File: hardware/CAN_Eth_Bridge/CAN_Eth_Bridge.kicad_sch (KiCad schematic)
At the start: 25 parts, among them J102 Global LV and CAN, J105 Conn_02x05_Odd_Even, J106 uart, SW101 SW_Push, U101 MCP2542FDxMF, U103 XMSM0G3507SDGS28R

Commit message: long 88 can stick
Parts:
- removed F101: ~1A, Fuse:Fuseholder_Blade_Mini_Keystone_3568, symbol Device:Fuse_Small
- removed J105: Conn_02x05_Odd_Even, Connector_PinHeader_1.27mm:PinHeader_2x05_P1.27mm_Vertical_SMD, symbol Connector_Generic:Conn_02x05_Odd_Even
- removed J106: uart, Connector_PinHeader_2.54mm:PinHeader_1x03_P2.54mm_Vertical, symbol Connector:Conn_01x03_Pin
- added C101, C102, C103: 220n, Capacitor_SMD:C_0805_2012Metric_Pad1.18x1.45mm_HandSolder, symbol Device:C_Small
- added D101: TS4148, Diode_SMD:D_0805_2012Metric_Pad1.15x1.40mm_HandSolder, symbol Device:D_Small
- added FL102: Choke_CommonMode_FerriteCore_1243, Inductor_SMD:L_CommonModeChoke_Coilcraft_1812CAN, symbol Filter:Choke_CommonMode_FerriteCore_1243
- added J101: Conn_01x05_Pin, Connector_PinHeader_2.54mm:PinHeader_1x05_P2.54mm_Vertical, symbol Connector:Conn_01x05_Pin
- added SW102: SW_DIP_x06, Button_Switch_SMD:SW_DIP_SPSTx06_Slide_Copal_CHS-06B_W7.62mm_P1.27mm, symbol Switch:SW_DIP_x06
- added U102: AP7384-50SA, Package_TO_SOT_SMD:SOT-23-3, symbol Regulator_Linear:AP7384-50SA
- added U104: AP7381-33SA-7, Package_TO_SOT_SMD:SOT-23, symbol Regulator_Linear:AP7381-33SA-7
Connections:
- net GLV- is gone; now on net GND: J102.2 (Pin_2)
- net +3.3V: now also U103.7 (VDD), C101.1, U104.2 (VO)
- net +5V: now also C102.1, U102.2 (VO)
- net GLV+: now also D101.2 (A)
- net GND: now also U103.8 (VSS), C101.2, C102.2, C103.2, J101.1 (Pin_1), U102.3 (GND), U104.3 (GND)
- net G_CAN+: now also FL102.1; no longer U101.7 (CANH)
- net G_CAN-: now also FL102.4; no longer U101.6 (CANL)
- net XDS_RXD: now also J101.3 (Pin_3)
- net XDS_TCK_SWDCLK: now also U103.23 (PA20/SWCLK), J101.5 (Pin_5)
- net XDS_TMS_SWDIO: now also U103.22 (PA19/SWDIO), J101.4 (Pin_4)
- net XDS_TXD: now also J101.2 (Pin_2)
- net vcore: now also U103.3 (VCORE)
- net at R112.1, SW101.1: now also U103.6 (NRST)
- net at U103.9 (PA2_/_ROSC): now also R111.2
- new net: C103.1, D101.1 (K), U102.1 (VI), U104.1 (VI)
- new net: FL102.3, U101.6 (CANL)
- new net: FL102.2, U101.7 (CANH)
- no-connect marks 4 -> 0
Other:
- removed sheet GLV PSU
- note added: "PSU"
- note removed: "- LV only. no HV present - (10,35]VDC GLV working - swap relays for >12VDC operation - IL assumed to share GLV GND - IL sense diode set for ~12VDC"
- note removed: "PWR"
- note removed: "SWD fish"
- moved on the sheet: C104, D103, D104, D105, D106, J102, R107, R108, R109, R110, U101, U103

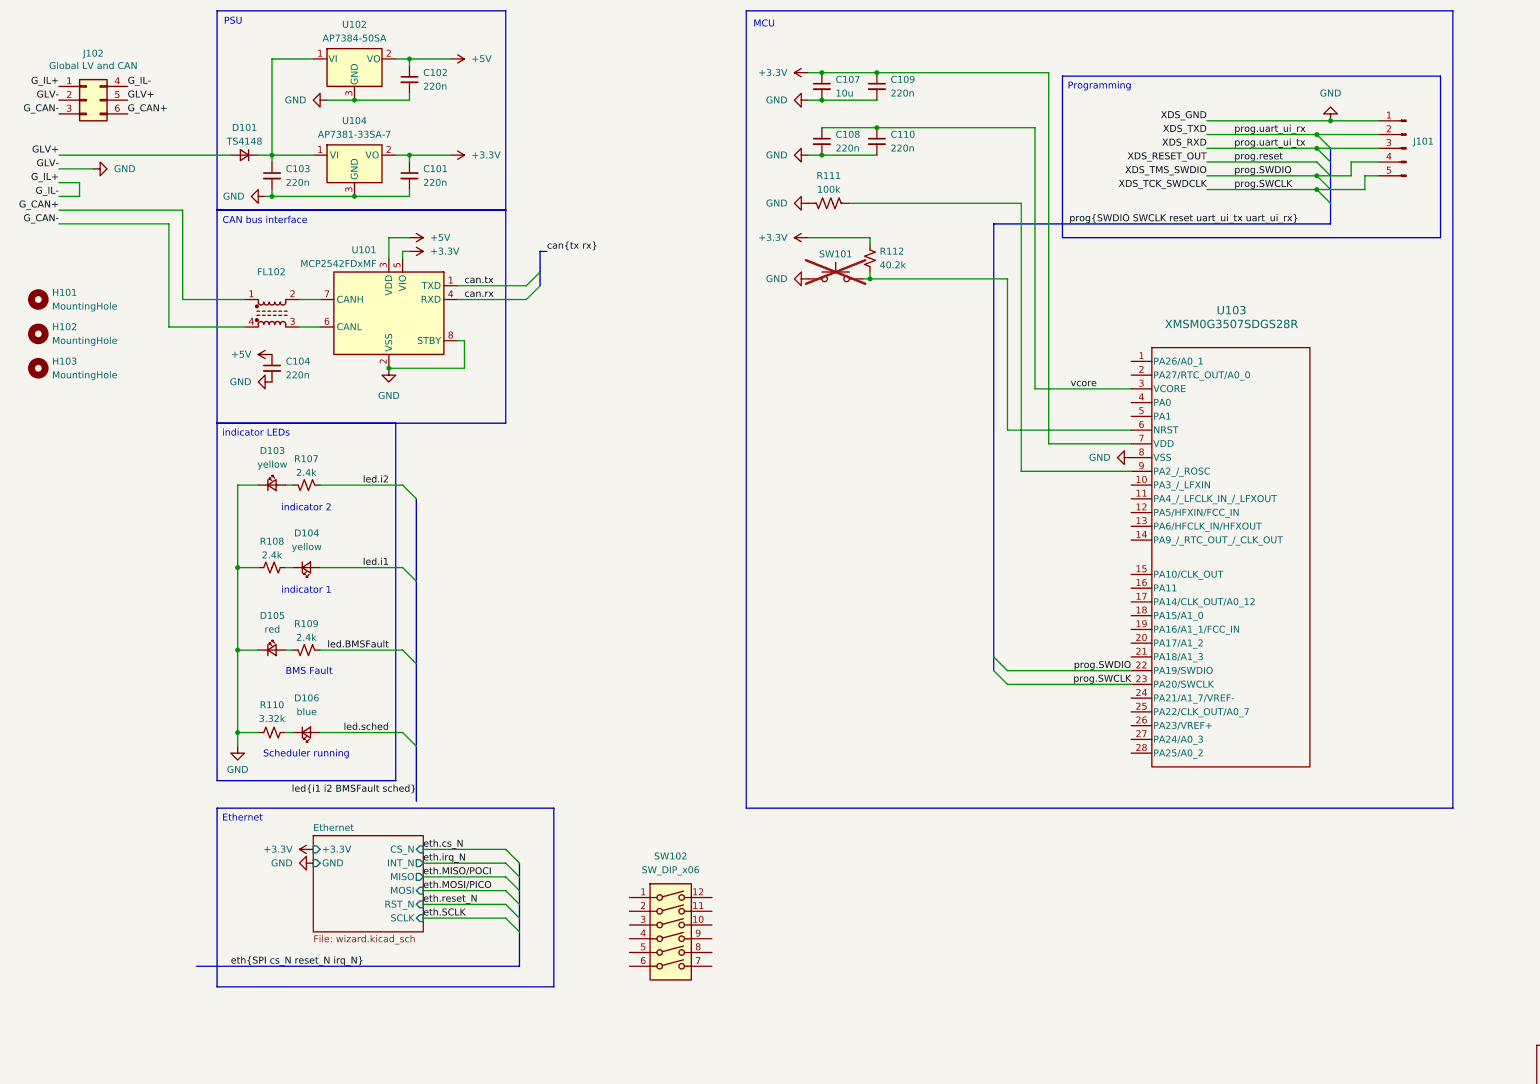
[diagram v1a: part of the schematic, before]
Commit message: shuffled
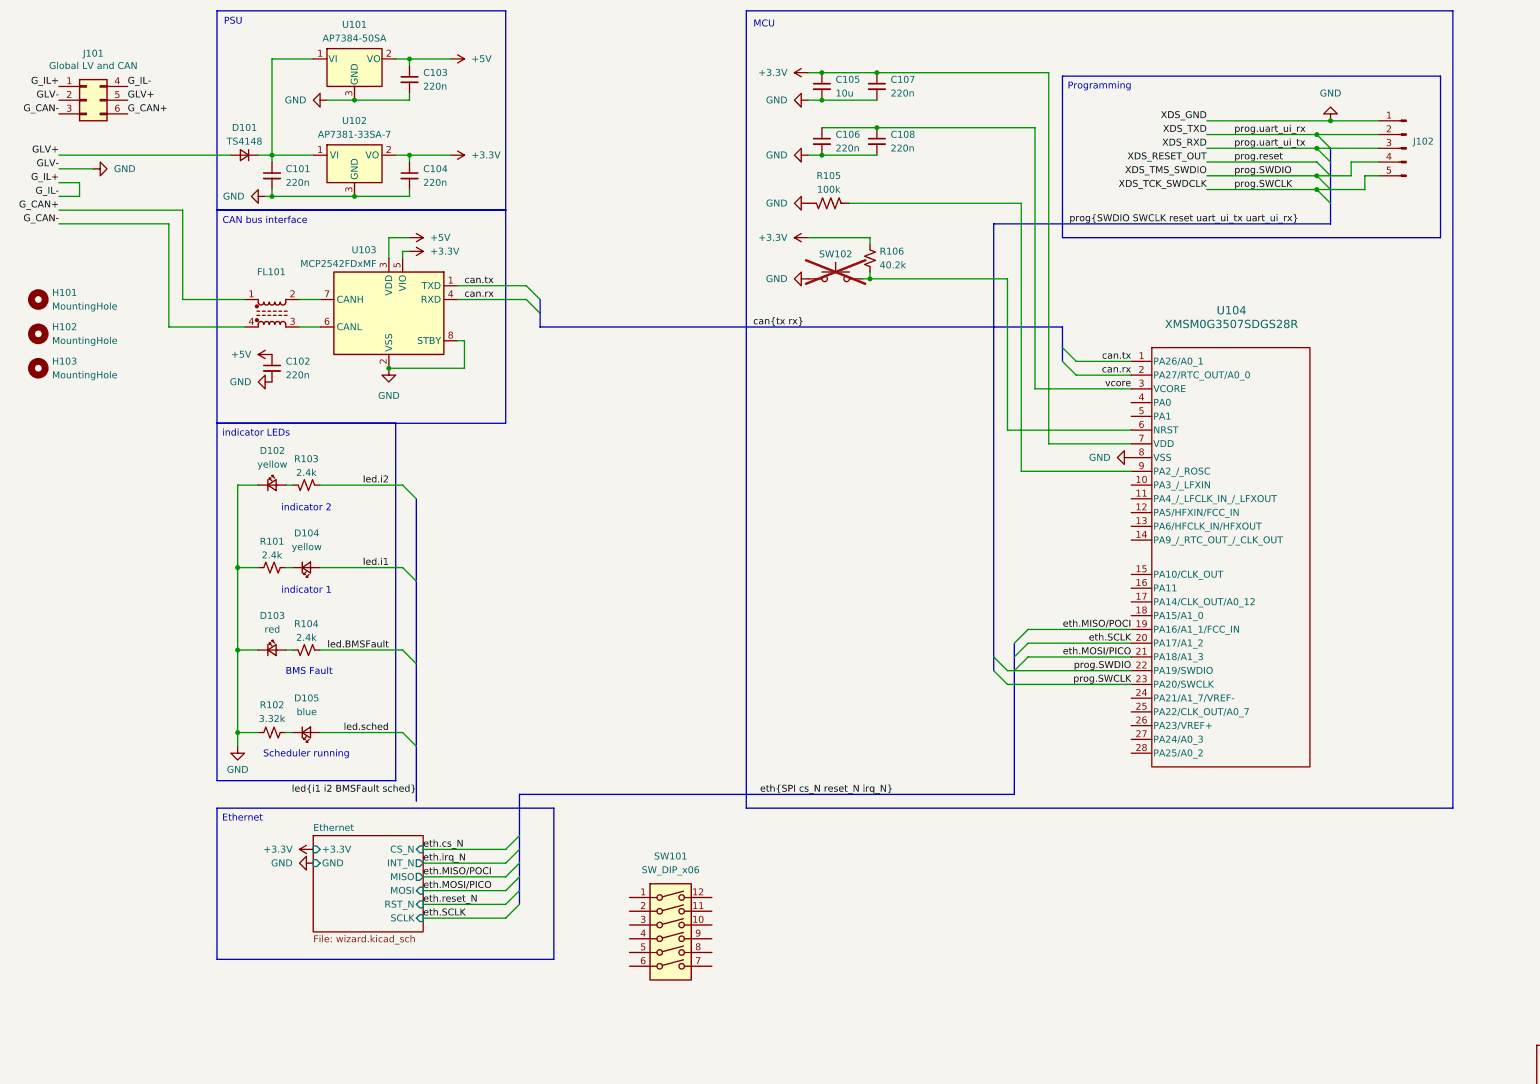
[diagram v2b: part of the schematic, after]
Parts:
- renumbered C103 to C101, C104 to C102, C102 to C103, C101 to C104, C107 to C105, C108 to C106, C109 to C107, C110 to C108, D103 to D102, D105 to D103, D106 to D105, FL102 to FL101, J102 to J101, J101 to J102, R108 to R101, R110 to R102, R107 to R103, R109 to R104, R111 to R105, R112 to R106, SW102 to SW101, SW101 to SW102, U102 to U101, U104 to U102, U101 to U103, U103 to U104
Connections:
- net can.rx: now also U104.2 (PA27/RTC_OUT/A0_0)
- net can.tx: now also U104.1 (PA26/A0_1)
- net eth.MISO/POCI: now also U104.19 (PA16/A1_1/FCC_IN)
- net eth.MOSI/PICO: now also U104.21 (PA18/A1_3)
- net eth.SCLK: now also U104.20 (PA17/A1_2)
